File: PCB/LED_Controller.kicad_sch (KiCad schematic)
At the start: 30 parts, among them J1 Barrel_Jack, J2 Conn_01x06_Female, J4 Add. LED Strip, J7 Conn_01x02, U1 ESP32-PICO-D4, U2 AP62200, U3 NCP1117-5.0_SOT223, U4 74LVCH2T45DC

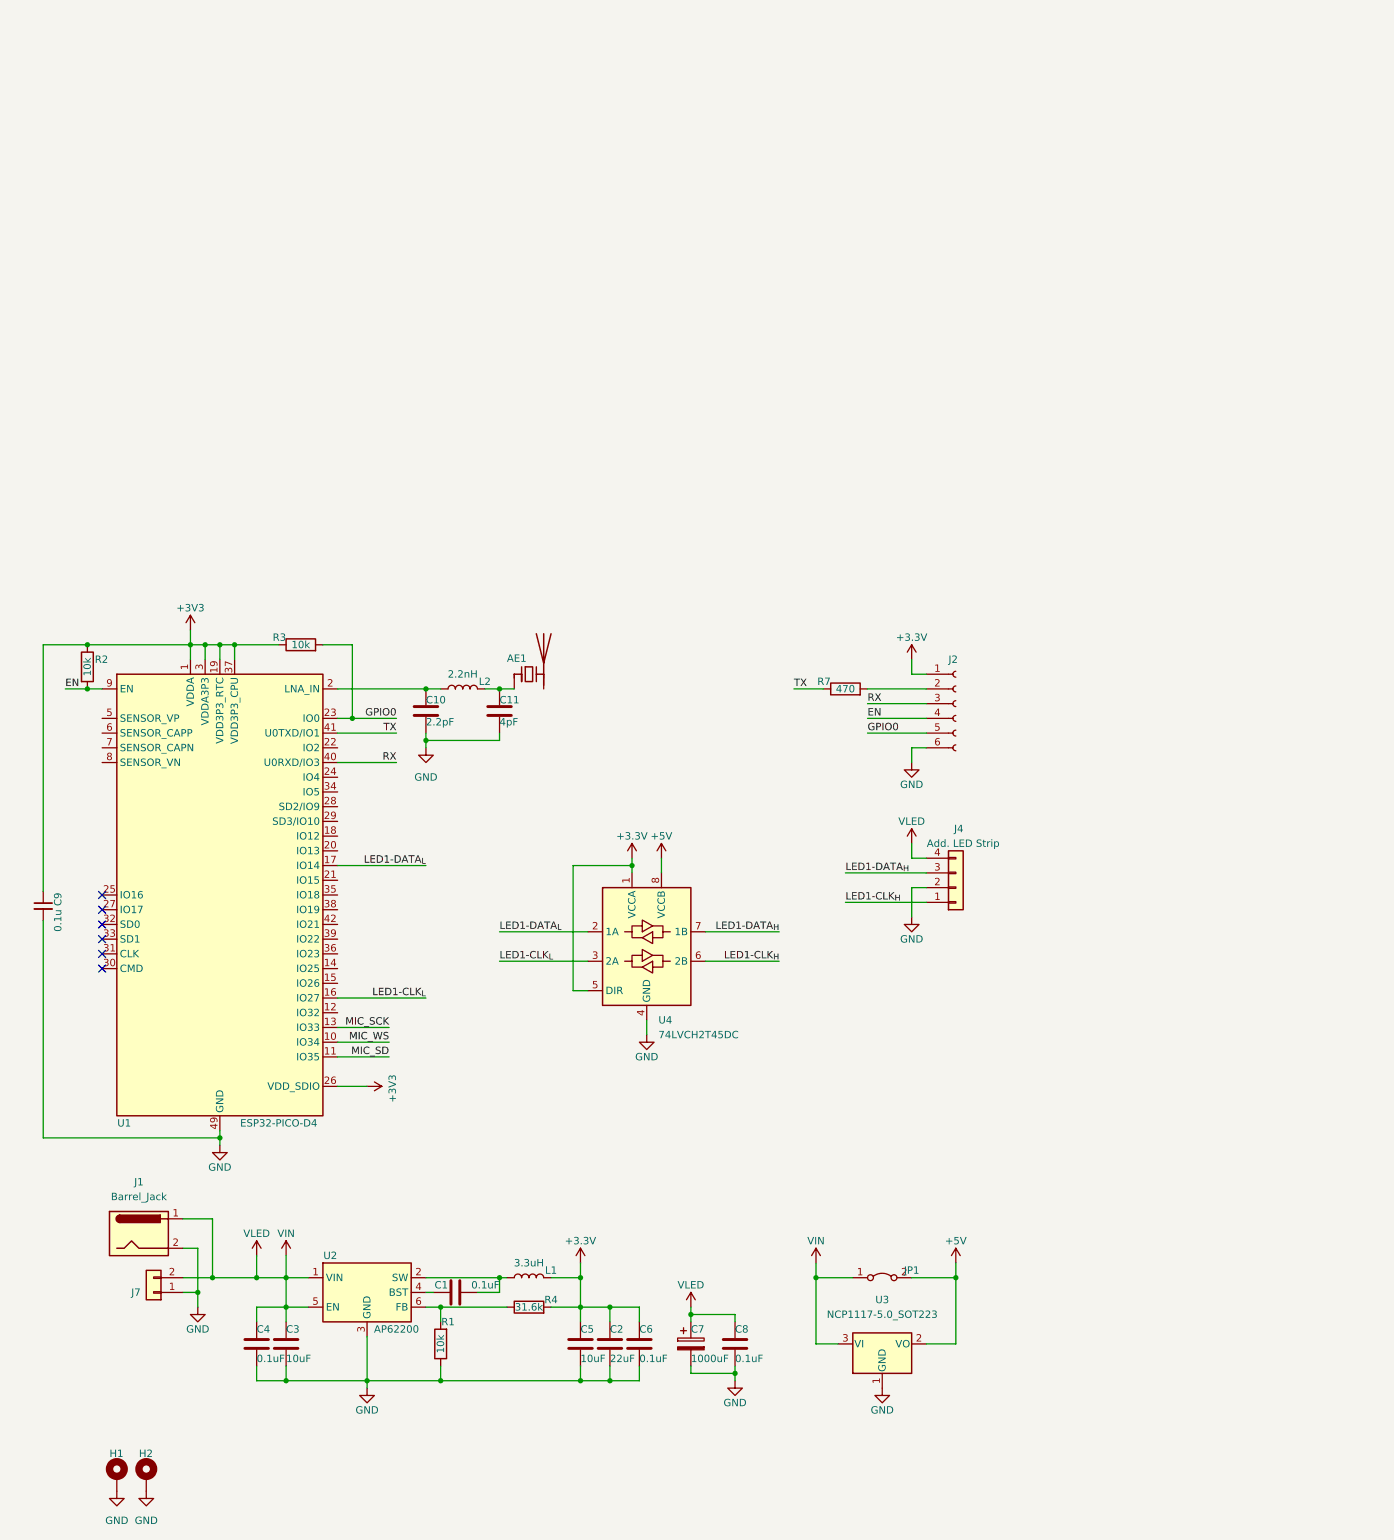
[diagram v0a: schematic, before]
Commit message: Started work on V3 of PCB
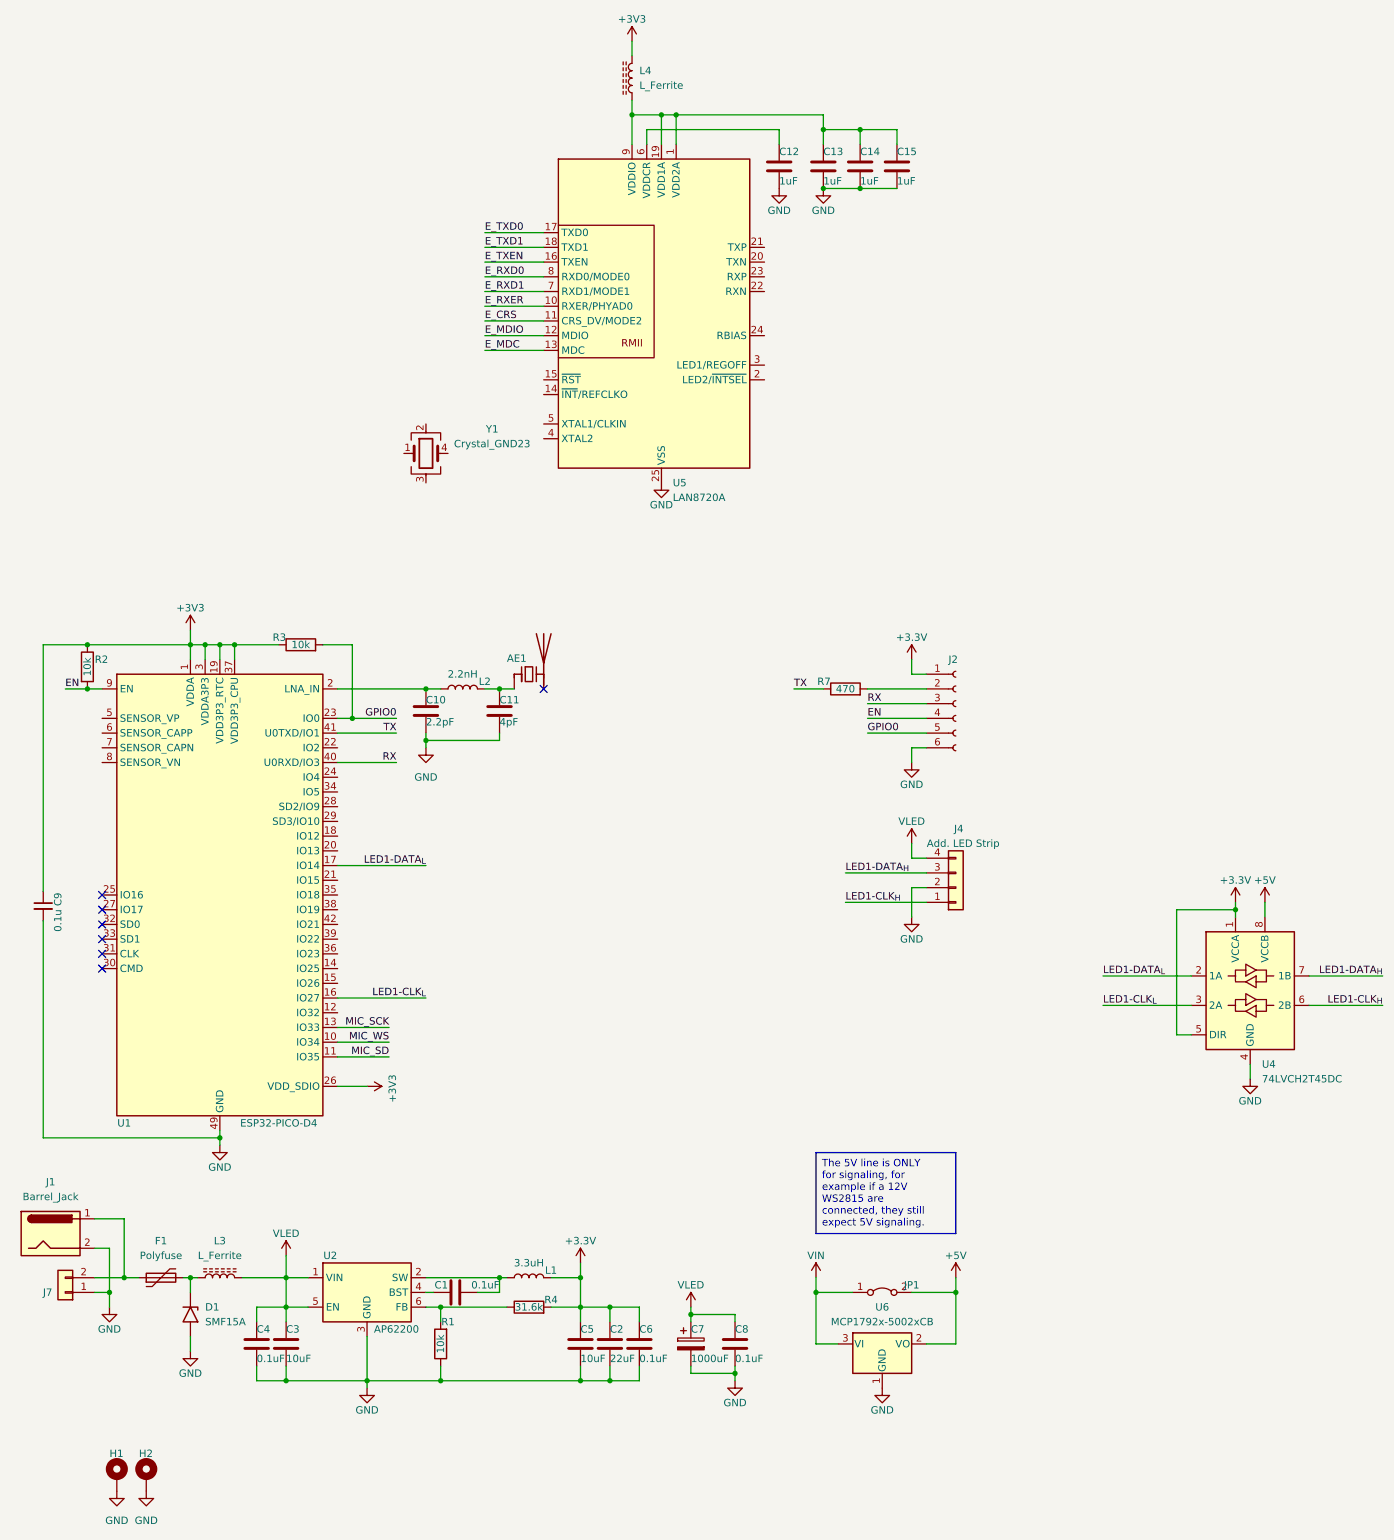
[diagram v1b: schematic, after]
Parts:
- removed U3: NCP1117-5.0_SOT223, Package_TO_SOT_SMD:SOT-223-3_TabPin2, symbol Regulator_Linear:NCP1117-5.0_SOT223
- added C12, C13, C14, C15: 1uF, symbol Device:C
- added D1: SMF15A, Diode_SMD:D_SMF, symbol Diode:SMF15A
- added F1: Polyfuse, symbol Device:Polyfuse
- added L3, L4: L_Ferrite, symbol Device:L_Ferrite
- added U5: LAN8720A, Package_DFN_QFN:VQFN-24-1EP_4x4mm_P0.5mm_EP2.5x2.5mm_ThermalVias, symbol Interface_Ethernet:LAN8720A
- added U6: MCP1792x-5002xCB, Package_TO_SOT_SMD:SOT-23, symbol Regulator_Linear:MCP1792x-5002xCB
- added Y1: Crystal_GND23, symbol Device:Crystal_GND23
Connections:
- net +3V3: now also L4.2
- net +5V: now also U6.2 (VO)
- net GND: now also C12.2, C13.2, C14.2, C15.2, D1.2 (A2), U5.25 (VSS), U6.1 (GND)
- net VIN: now also U6.3 (VI); no longer C3.1, C4.1, C7.1, C8.1, J1.1, J4.4 (Pin_4), J7.2 (Pin_2), U2.1 (VIN), U2.5 (EN)
- new net: C13.1, C14.1, C15.1, L4.1, U5.1 (VDD2A), U5.19 (VDD1A), U5.9 (VDDIO)
- new net: F1.1, J1.1, J7.2 (Pin_2)
- new net: D1.1 (A1), F1.2, L3.1
- new net: C12.1, U5.6 (VDDCR)
- new net E_CRS: U5.11 (CRS_DV/MODE2)
- new net E_MDC: U5.13 (MDC)
- new net E_MDIO: U5.12 (MDIO)
- new net E_RXD0: U5.8 (RXD0/MODE0)
- new net E_RXD1: U5.7 (RXD1/MODE1)
- new net E_RXER: U5.10 (RXER/PHYAD0)
- new net E_TXD0: U5.17 (TXD0)
- new net E_TXD1: U5.18 (TXD1)
- new net E_TXEN: U5.16 (TXEN)
- new net VLED: C3.1, C4.1, C7.1, C8.1, J4.4 (Pin_4), L3.2, U2.1 (VIN), U2.5 (EN)
- no-connect marks 6 -> 7
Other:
- moved on the sheet: J1, J7, JP1, U4
